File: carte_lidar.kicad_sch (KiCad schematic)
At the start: 26 parts, among them J1 Conn_01x03_Pin, J2 Conn_01x02_Pin, J3 Conn_01x05_Socket, J4 Conn_01x02, J5 Conn_01x04_Socket, U1 TPS54302, U2 Pico

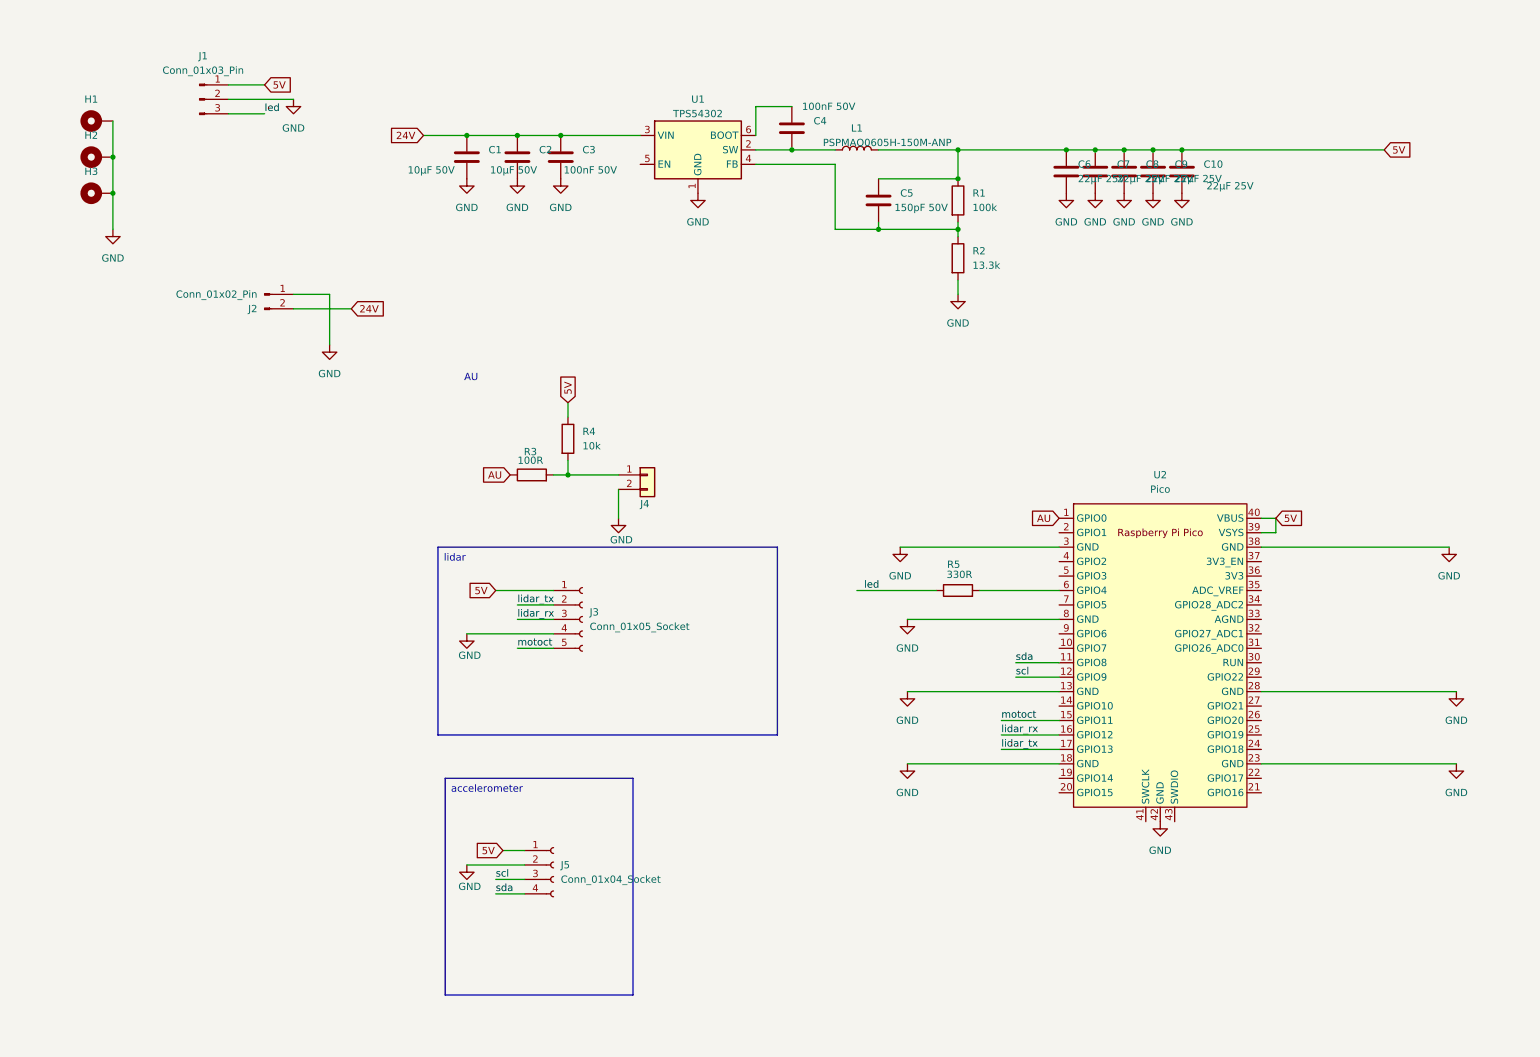
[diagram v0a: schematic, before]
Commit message: update all
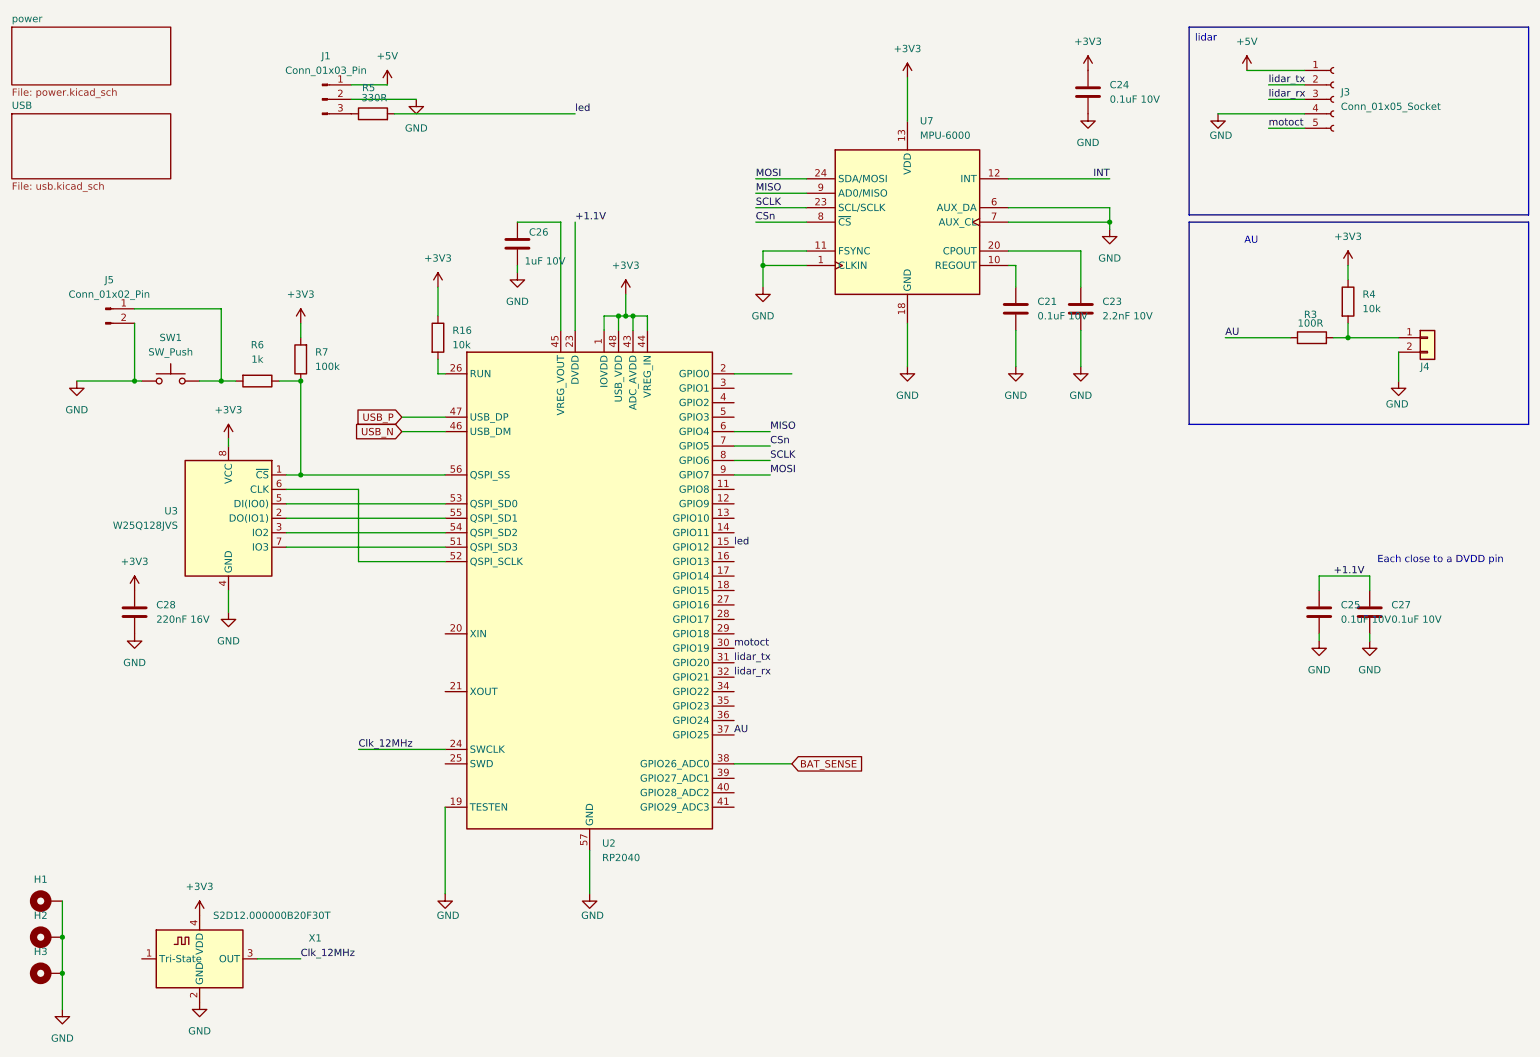
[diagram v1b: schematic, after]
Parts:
- removed C1, C2: 10µF 50V, Capacitor_SMD:C_1206_3216Metric, symbol Device:C
- removed C10, C6, C7, C8, C9: 22µF 25V, Capacitor_SMD:C_0805_2012Metric, symbol Device:C
- removed C3: 100nF 50V, Capacitor_SMD:C_0805_2012Metric, symbol Device:C
- removed C4: 100nF 50V, Capacitor_SMD:C_0402_1005Metric, symbol Device:C
- removed C5: 150pF 50V, Capacitor_SMD:C_1206_3216Metric, symbol Device:C
- removed J2: Conn_01x02_Pin, Connector_AMASS:AMASS_XT30U-F_1x02_P5.0mm_Vertical, symbol Connector:Conn_01x02_Pin
- removed J5: Conn_01x04_Socket, Connector_PinSocket_2.54mm:PinSocket_1x04_P2.54mm_Vertical, symbol Connector:Conn_01x04_Socket
- removed L1: PSPMAQ0605H-150M-ANP, 7Robot_lib:Prod_Tech_7.1x6.6mm, symbol Device:L
- removed R1: 100k, Resistor_SMD:R_0603_1608Metric, symbol Device:R
- removed R2: 13.3k, Resistor_SMD:R_0603_1608Metric, symbol Device:R
- removed U1: TPS54302, Package_TO_SOT_SMD:SOT-23-6, symbol Regulator_Switching:TPS54302
- removed U2: Pico, MCU_RaspberryPi_and_Boards:RPi_Pico_SMD_TH, symbol MCU_RaspberryPi_and_Boards:Pico
- added C21, C24, C25, C27: 0.1uF 10V, Capacitor_SMD:C_0402_1005Metric, symbol Device:C
- added C23: 2.2nF 10V, Capacitor_SMD:C_0402_1005Metric, symbol Device:C
- added C26: 1uF 10V, Capacitor_SMD:C_0402_1005Metric, symbol Device:C
- added C28: 220nF 16V, Capacitor_SMD:C_0402_1005Metric, symbol Device:C
- added J5: Conn_01x02_Pin, Connector_PinHeader_2.54mm:PinHeader_1x02_P2.54mm_Vertical, symbol Connector:Conn_01x02_Pin
- added R16: 10k, Capacitor_SMD:C_0402_1005Metric, symbol Device:R
- added R6: 1k, Resistor_SMD:R_0402_1005Metric, symbol Device:R
- added R7: 100k, Resistor_SMD:R_0402_1005Metric, symbol Device:R
- added SW1: SW_Push, Button_Switch_SMD:SW_SPST_B3U-1000P, symbol Switch:SW_Push
- added U2: RP2040, Package_DFN_QFN:QFN-56-1EP_7x7mm_P0.4mm_EP3.2x3.2mm_ThermalVias, symbol MCU_RaspberryPi:RP2040
- added U3: W25Q128JVS, Package_SO:SOIC-8_5.23x5.23mm_P1.27mm, symbol Memory_Flash:W25Q128JVS
- added U7: MPU-6000, Sensor_Motion:InvenSense_QFN-24_4x4mm_P0.5mm, symbol Sensor_Motion:MPU-6000
- added X1: S2D12.000000B20F30T, Oscillator:Oscillator_SMD_ECS_2520MV-xxx-xx-4Pin_2.5x2.0mm, symbol Oscillator:ECS-2520MV-xxx-xx
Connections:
- net AU: now also U2.37 (GPIO25)
- net GND: now also C21.2, C23.2, C24.2, C25.2, C26.2, C27.2, C28.2, J5.2 (Pin_2), SW1.1, U2.19 (TESTEN), U2.57 (GND), U3.4 (GND), U7.1 (CLKIN), U7.11 (FSYNC), U7.18 (GND), U7.6 (AUX_DA), U7.7 (AUX_CL), X1.2 (GND)
- net led: now also R5.2, U2.15 (GPIO12); no longer J1.3 (Pin_3), R5.1
- net lidar_rx: now also U2.32 (GPIO21)
- net lidar_tx: now also U2.31 (GPIO20)
- net motoct: now also U2.30 (GPIO19)
- net 5V renamed +5V
- net +5V: no longer R4.1
- new net: C23.1, U7.20 (CPOUT)
- new net: J1.3 (Pin_3), R5.1
- new net: R16.2, U2.26 (RUN)
- new net: C26.1, U2.45 (VREG_VOUT)
- new net: U2.51 (QSPI_SD3), U3.7 (IO3)
- new net: U2.52 (QSPI_SCLK), U3.6 (CLK)
- new net: U2.53 (QSPI_SD0), U3.5 (DI(IO0))
- new net: U2.54 (QSPI_SD2), U3.3 (IO2)
- new net: U2.55 (QSPI_SD1), U3.2 (DO(IO1))
- new net: R6.1, R7.1, U2.56 (QSPI_SS), U3.1 (~{CS})
- new net: J5.1 (Pin_1), R6.2, SW1.2
- new net: C21.1, U7.10 (REGOUT)
- new net +1.1V: C25.1, C27.1, U2.23 (DVDD), U2.50 (DVDD)
- new net +3V3: C24.1, C28.1, R16.1, R4.1, R7.2, U2.1 (IOVDD), U2.10 (IOVDD), U2.22 (IOVDD), U2.33 (IOVDD), U2.42 (IOVDD), U2.43 (ADC_AVDD), U2.44 (VREG_IN), U2.48 (USB_VDD), U2.49 (IOVDD), U3.8 (VCC), U7.13 (VDD), X1.4 (VDD)
- new net BAT_SENSE: U2.38 (GPIO26_ADC0)
- new net CSn: U2.7 (GPIO5), U7.8 (~{CS})
- new net Clk_12MHz: U2.24 (SWCLK), X1.3 (OUT)
- new net INT: U7.12 (INT)
- new net MISO: U2.6 (GPIO4), U7.9 (AD0/MISO)
- new net MOSI: U2.9 (GPIO7), U7.24 (SDA/MOSI)
- new net SCLK: U2.8 (GPIO6), U7.23 (SCL/SCLK)
- new net USB_N: U2.46 (USB_DM)
- new net USB_P: U2.47 (USB_DP)
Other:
- added sheet USB (usb.kicad_sch)
- added sheet power (power.kicad_sch)
- note added: "Each close to a DVDD pin"
- moved on the sheet: H1, H2, H3, J1, J3, J4, R3, R4
